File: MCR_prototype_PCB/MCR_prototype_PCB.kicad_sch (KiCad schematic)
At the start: 4 parts, among them J0 Conn_02x20_Odd_Even

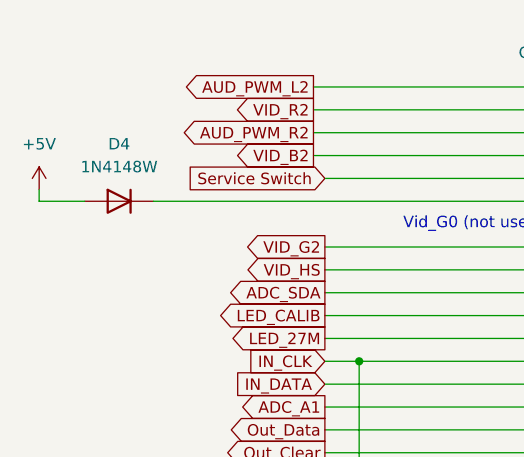
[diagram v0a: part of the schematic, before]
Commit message: Add files via upload
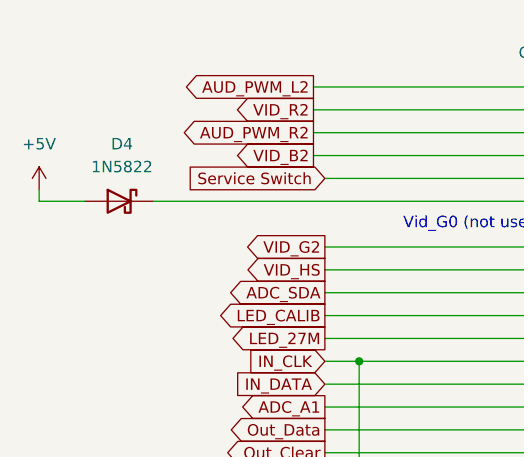
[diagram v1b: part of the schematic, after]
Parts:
- removed D4: 1N4148W, Diode_SMD:D_SOD-123, symbol Diode:1N4148W
- added D4: 1N5822, Diode_THT:D_DO-201AD_P15.24mm_Horizontal, symbol Diode:1N5822
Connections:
- net +5V: now also D4.2 (A)
- net at J0.11 (Pin_11): now also D4.1 (K)
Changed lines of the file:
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@@
+	)
+	(symbol
+		(lib_id "Diode:1N5822")
+		(at 90.17 71.12 0)
+		(mirror y)
+		(unit 1)
+		(body_style 1)
+		(exclude_from_sim no)
+		(in_bom yes)
+		(on_board yes)
+		(in_pos_files yes)
+		(dnp no)
+		(property "Reference" "D4"
+			(at 90.4875 64.77 0)
+			(show_name no)
+			(do_not_autoplace no)
+			(effects
+				(font
+					(size 1.27 1.27)
+				)
+			)
+		)
+		(property "Value" "1N5822"
+			(at 90.4875 67.31 0)
+			(show_name no)
+			(do_not_autoplace no)
+			(effects
+				(font
+					(size 1.27 1.27)
+				)
+			)
+		)
+		(property "Footprint" "Diode_THT:D_DO-201AD_P15.24mm_Horizontal"
+			(at 90.17 75.565 0)
+			(hide yes)
+			(show_name no)
+			(do_not_autoplace no)
+			(effects
+				(font
+					(size 1.27 1.27)
+				)
+			)
+		)
+		(property "Datasheet" "http://www.vishay.com/docs/88526/1n5820.pdf"
+			(at 90.17 71.12 0)
+			(hide yes)
+			(show_name no)
+			(do_not_autoplace no)
+			(effects
+				(font
+					(size 1.27 1.27)
+				)
+			)
+		)
+		(property "Description" "40V 3A Schottky Barrier Rectifier Diode, DO-201AD"
+			(at 90.17 71.12 0)
+			(hide yes)
+			(show_name no)
+			(do_not_autoplace no)
+			(effects
+				(font
+					(size 1.27 1.27)
+				)
+			)
+		)
+		(pin "1"
+		)
+		(pin "2"
+		)
+		(instances
+			(project "MCR_prototype_PCB"
+				(path "/b80aa942-218c-4c9e-b346-37092f7eeec3"
+					(reference "D4")
+					(unit 1)
+				)
+			)
+		)
 	)
 	(symbol
@@
 					(unit 1)
 				)
-			)
-		)
-	)
-	(symbol
-		(lib_id "Diode:1N4148W")
-		(at 90.17 71.12 0)
-		(mirror y)
-		(unit 1)
-		(body_style 1)
-		(exclude_from_sim no)
-		(in_bom yes)
-		(on_board yes)
-		(in_pos_files yes)
-		(dnp no)
-		(property "Reference" "D4"
-			(at 90.17 64.77 0)
-			(show_name no)
-			(do_not_autoplace no)
-			(effects
-				(font
-					(size 1.27 1.27)
-				)
-			)
-		)
-		(property "Value" "1N4148W"
-			(at 90.17 67.31 0)
-			(show_name no)
-			(do_not_autoplace no)
-			(effects
-				(font
-					(size 1.27 1.27)
-				)
-			)
-		)
-		(property "Footprint" "Diode_SMD:D_SOD-123"
-			(at 90.17 75.565 0)
-			(hide yes)
-			(show_name no)
-			(do_not_autoplace no)
-			(effects
-				(font
-					(size 1.27 1.27)
-				)
-			)
-		)
-		(property "Datasheet" "https://www.vishay.com/docs/85748/1n4148w.pdf"
-			(at 90.17 71.12 0)
-			(hide yes)
-			(show_name no)
-			(do_not_autoplace no)
-			(effects
-				(font
-					(size 1.27 1.27)
-				)
-			)
-		)
-		(property "Description" "75V 0.15A Fast Switching Diode, SOD-123"
-			(at 90.17 71.12 0)
-			(hide yes)
-			(show_name no)
-			(do_not_autoplace no)
-			(effects
-				(font
-					(size 1.27 1.27)
-				)
-			)
-		)
-		(property "Sim.Device" "D"
-			(at 90.17 71.12 0)
-			(hide yes)
-			(show_name no)
-			(do_not_autoplace no)
-			(effects
-				(font
-					(size 1.27 1.27)
-				)
-			)
-		)
-		(property "Sim.Pins" "1=K 2=A"
-			(at 90.17 71.12 0)
-			(hide yes)
-			(show_name no)
-			(do_not_autoplace no)
-			(effects
-				(font
-					(size 1.27 1.27)
-				)
-			)
-		)
-		(pin "1"
-		)
-		(pin "2"
-		)
-		(instances
-			(project "MCR_prototype_PCB"
-				(path "/b80aa942-218c-4c9e-b346-37092f7eeec3"
-					(reference "D4")
-					(unit 1)
-				)

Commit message: Production/schematics for 10/10/26 first board run
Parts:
- D4: LCSC (none) -> C2476
- J0: LCSC (none) -> C2897421
- TP5, TP6: footprint TestPoint:TestPoint_Loop_D1.80mm_Drill1.0mm_Beaded -> TestPoint:TestPoint_Pad_1.5x1.5mm
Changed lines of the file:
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@@
 			)
 		)
-		(property "Footprint" "TestPoint:TestPoint_Loop_D1.80mm_Drill1.0mm_Beaded"
+		(property "Footprint" "TestPoint:TestPoint_Pad_1.5x1.5mm"
 			(at 172.72 116.84 0)
 			(hide yes)
@@
 		)
 		(property "Description" "test point"
+			(at 167.64 116.84 0)
+			(hide yes)
+			(show_name no)
+			(do_not_autoplace no)
+			(effects
+				(font
+					(size 1.27 1.27)
+				)
+			)
+		)
+		(property "KLC_S3.3" ""
+			(at 167.64 116.84 0)
+			(hide yes)
+			(show_name no)
+			(do_not_autoplace no)
+			(effects
+				(font
+					(size 1.27 1.27)
+				)
+			)
+		)
+		(property "KLC_S5.1" ""
+			(at 167.64 116.84 0)
+			(hide yes)
+			(show_name no)
+			(do_not_autoplace no)
+			(effects
+				(font
+					(size 1.27 1.27)
+				)
+			)
+		)
+		(property "LCSC" ""
 			(at 167.64 116.84 0)
 			(hide yes)
@@
 			)
 		)
+		(property "LCSC" "C2476"
+			(at 90.17 71.12 0)
+			(hide yes)
+			(show_name no)
+			(do_not_autoplace no)
+			(effects
+				(font
+					(size 1.27 1.27)
+				)
+			)
+		)
+		(property "KLC_S3.3" ""
+			(at 90.17 71.12 0)
+			(hide yes)
+			(show_name no)
+			(do_not_autoplace no)
+			(effects
+				(font
+					(size 1.27 1.27)
+				)
+			)
+		)
+		(property "KLC_S5.1" ""
+			(at 90.17 71.12 0)
+			(hide yes)
+			(show_name no)
+			(do_not_autoplace no)
+			(effects
+				(font
+					(size 1.27 1.27)
+				)
+			)
+		)
 		(pin "1"
 		)
@@
 			)
 		)
-		(property "Footprint" "TestPoint:TestPoint_Loop_D1.80mm_Drill1.0mm_Beaded"
+		(property "Footprint" "TestPoint:TestPoint_Pad_1.5x1.5mm"
 			(at 121.92 113.03 0)
 			(hide yes)
@@
 		)
 		(property "Description" "test point"
+			(at 116.84 113.03 0)
+			(hide yes)
+			(show_name no)
+			(do_not_autoplace no)
+			(effects
+				(font
+					(size 1.27 1.27)
+				)
+			)
+		)
+		(property "KLC_S3.3" ""
+			(at 116.84 113.03 0)
+			(hide yes)
+			(show_name no)
+			(do_not_autoplace no)
+			(effects
+				(font
+					(size 1.27 1.27)
+				)
+			)
+		)
+		(property "KLC_S5.1" ""
+			(at 116.84 113.03 0)
+			(hide yes)
+			(show_name no)
+			(do_not_autoplace no)
+			(effects
+				(font
+					(size 1.27 1.27)
+				)
+			)
+		)
+		(property "LCSC" ""
 			(at 116.84 113.03 0)
 			(hide yes)
@@
 			(at 143.51 81.28 0)
 			(hide yes)
+			(show_name no)
+			(do_not_autoplace no)
+			(effects
+				(font
+					(size 1.27 1.27)
+				)
+			)
+		)
+		(property "KLC_S3.3" ""
+			(at 143.51 81.28 0)
+			(hide yes)
+			(show_name no)
+			(do_not_autoplace no)
+			(effects
+				(font
+					(size 1.27 1.27)
+				)
+			)
+		)
+		(property "KLC_S5.1" ""
+			(at 143.51 81.28 0)
+			(hide yes)
+			(show_name no)
+			(do_not_autoplace no)
+			(effects
+				(font
+					(size 1.27 1.27)
+				)
+			)
+		)
+		(property "LCSC" "C2897421"
+			(at 143.51 81.28 0)
+			(hide yes)
